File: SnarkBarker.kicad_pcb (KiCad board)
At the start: 2 copper layers, 231.1 x 106.7 mm, 199 parts, among them J1 Bus_ISA_8bit, J2 Bracket Mount, P1 Joystick/MIDI, P2 L7809, T1 2N3904, T2 2N3904, U1 NE558, U10 YM3014B, U11 NJM3403A, U12 MC1408_DIP, U13 805X, U14 SAA1099, U15 SAA1099, U16 74LS08, U17 74LS139, U18 74LS374, U19 74LS374, U2 74LS245, U20 74LS74, U21 74LS125, U22 74LS74, U23 74LS74, U24 74LS32, U25 74LS08, U26 74LS74, U27 74LS32, U28 74LS08, U29 74LS14, U3 74LS244, U30 74LS32, U4 TEA2025B, U5 LM324, U6 LM393, U7 74LS138, U8 74LS138, U9 YM3812

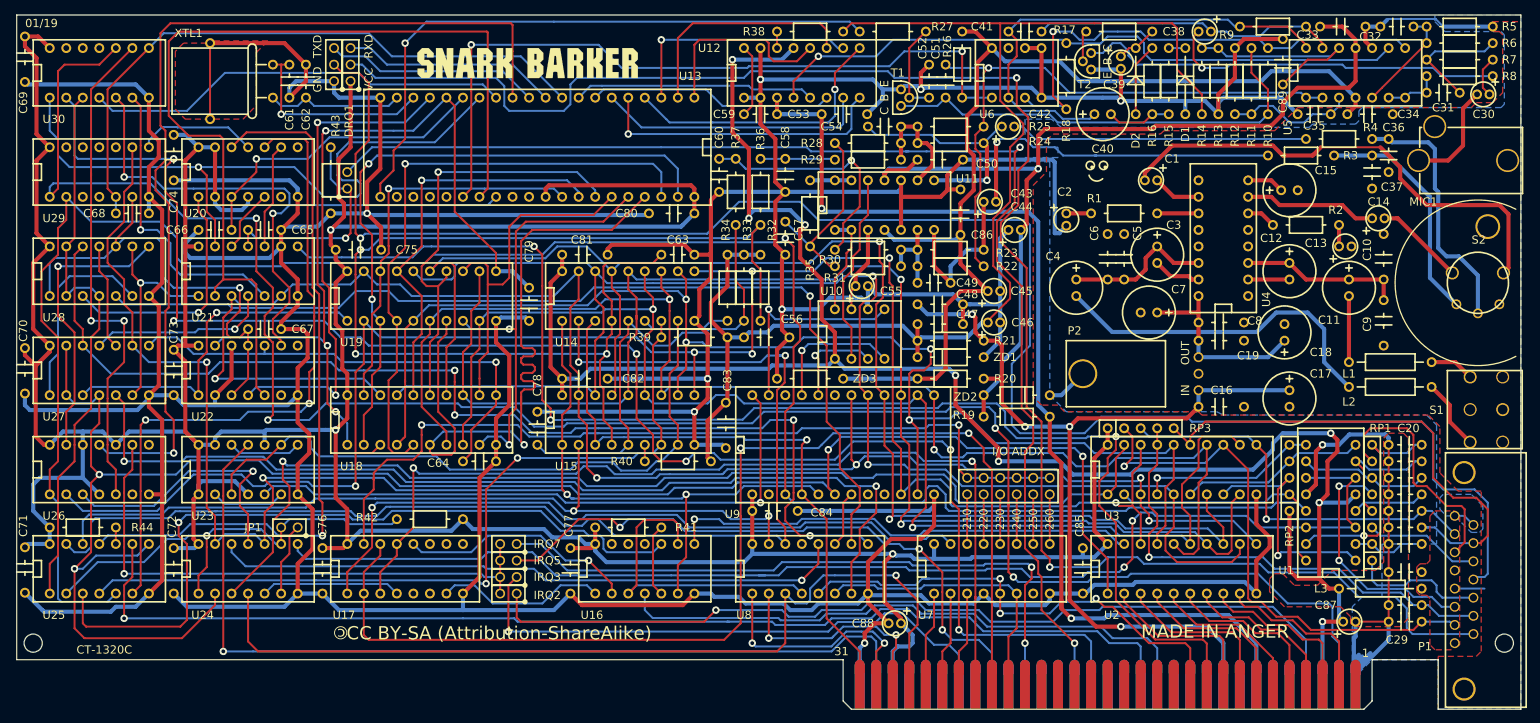
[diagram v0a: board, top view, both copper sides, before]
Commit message: Updating KICAD version files
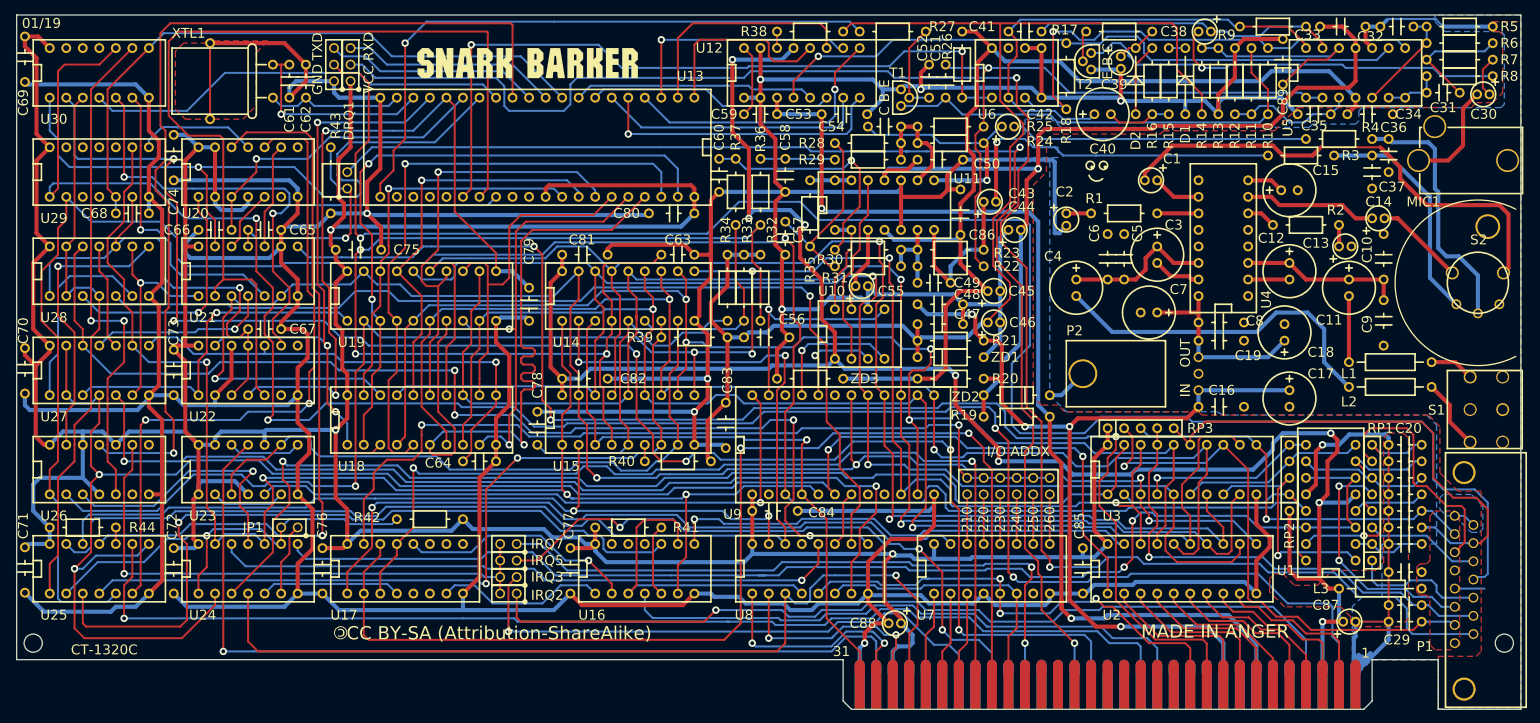
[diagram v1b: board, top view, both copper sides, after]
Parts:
- REF**: footprint Conn:MNT_KEYSTONE_9200 -> SoundBlaster:MNT_KEYSTONE_9200
- REF***: footprint Symbols:WEEE-Logo_8.4x12mm_SilkScreen -> SoundBlaster:WEEE-Logo_8.4x12mm_SilkScreen
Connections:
- net /CMS1-6_~CS renamed /CMS1-6_~{CS}
- net /CMS7-12_~CS renamed /CMS7-12_~{CS}
- net /DAV_~CS renamed /DAV_~{CS}
- net /DSPRD_~CS renamed /DSPRD_~{CS}
- net /DSPRST_~CS renamed /DSPRST_~{CS}
- net /DSPWR_~CS renamed /DSPWR_~{CS}
- net /FM_~CS renamed /FM_~{CS}
- net /JOYSTICK_~CS renamed /JOYSTICK_~{CS}
- net /~100000xxxx renamed /~{100000xxxx}
- net /~100jjjxxxx renamed /~{100jjjxxxx}
- net /~111000xxxx renamed /~{111000xxxx}
- net /~CARD_SELECTED renamed /~{CARD_SELECTED}
- net /~DACK1 renamed /~{DACK1}
- net /~DB_EN renamed /~{DB_EN}
- net /~DMAOUT renamed /~{DMAOUT}
- net /~DMA_EN renamed /~{DMA_EN}
- net /~DSP_READ renamed /~{DSP_READ}
- net /~DSP_WRITE renamed /~{DSP_WRITE}
- net /~IC renamed /~{IC}
- net /~IOR renamed /~{IOR}
- net /~IOW renamed /~{IOW}
- net /~ISA_RD renamed /~{ISA_RD}
- net /~ISA_WR renamed /~{ISA_WR}
- net /~RD renamed /~{RD}
- net /~RD_DAV renamed /~{RD_DAV}
- net /~RESET renamed /~{RESET}
- net /~WR renamed /~{WR}
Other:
- net class Default removed
